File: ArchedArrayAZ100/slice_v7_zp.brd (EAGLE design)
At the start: 196.4 x 249.7 mm, 118 parts

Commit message: added slice_v7 ArchedArray with 4 layers
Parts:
- removed F1: (no value), ZacksLib2:LITTLEFUSE_111_501
- moved U$1 8.00 mm to (140.0, 249.0)
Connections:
- removed net N$284: F1.P2_1, F1.P2_2, U$1.P$2
- net VCC: now also U$1.P$2; no longer F1.P1_1, F1.P1_2
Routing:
- net VCC: track 1271.0 -> 17.6 mm, vias 24 -> 1
- net N$284: track 11.3 -> 0.00 mm
- added copper zone on layer 2, net VCC

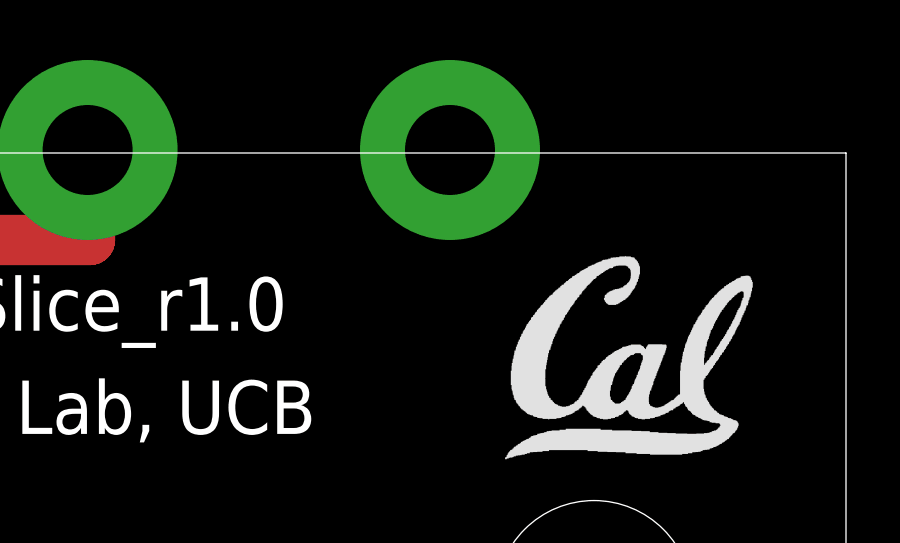
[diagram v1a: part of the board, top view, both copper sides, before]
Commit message: ArchedArray before moving board 6
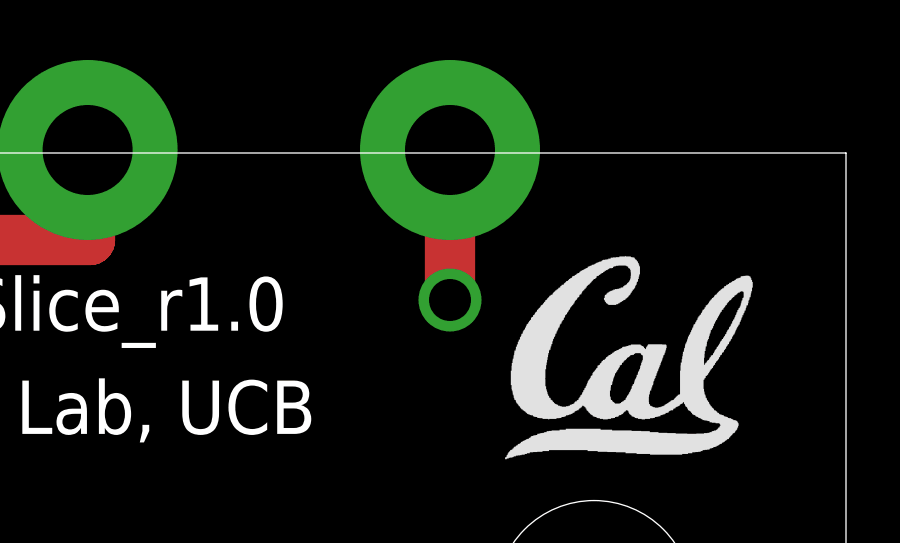
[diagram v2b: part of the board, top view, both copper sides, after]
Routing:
- net VCC: track 17.6 -> 78.7 mm
- net GND: track 617.8 -> 630.8 mm, vias 16 -> 17
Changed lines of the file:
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@@
 <wire x1="128" y1="246" x2="114.5" y2="246" width="1.6764" layer="1"/>
 <via x="114.5" y="246" extent="1-2" drill="1.4"/>
-<wire x1="114.5" y1="246" x2="114.5" y2="245" width="1.6764" layer="2"/>
+<wire x1="111" y1="226.365" x2="115.5" y2="226.365" width="1.6764" layer="2"/>
+<wire x1="115.5" y1="226.365" x2="115.5" y2="224.5" width="1.6764" layer="2"/>
+<wire x1="115.5" y1="224.5" x2="114.5" y2="224.5" width="1.6764" layer="2"/>
+<wire x1="114.5" y1="224.5" x2="114.5" y2="220" width="1.6764" layer="2"/>
+<wire x1="114.5" y1="220" x2="106" y2="220" width="1.6764" layer="2"/>
+<wire x1="106" y1="220" x2="106" y2="219.635" width="1.6764" layer="2"/>
+<wire x1="111" y1="242.365" x2="111" y2="242.5" width="1.6764" layer="2"/>
+<wire x1="111" y1="242.5" x2="114.5" y2="242.5" width="1.6764" layer="2"/>
+<wire x1="114.5" y1="242.5" x2="114.5" y2="246" width="1.6764" layer="2"/>
+<wire x1="111" y1="234.365" x2="114.5" y2="234.365" width="1.6764" layer="2"/>
+<wire x1="114.5" y1="234.365" x2="114.5" y2="242.5" width="1.6764" layer="2"/>
+<wire x1="111" y1="226.365" x2="114.5" y2="226.365" width="1.6764" layer="2"/>
+<wire x1="114.5" y1="226.365" x2="114.5" y2="234.365" width="1.6764" layer="2"/>
 <wire x1="62.635" y1="182" x2="62.635" y2="188.5" width="0" layer="19" extent="1-1"/>
 <wire x1="66.635" y1="194.5" x2="62.635" y2="188.5" width="0" layer="19" extent="1-1"/>
@@
 <wire x1="94" y1="219.635" x2="88" y2="218.365" width="0" layer="19" extent="1-1"/>
 <wire x1="100" y1="219.635" x2="94" y2="219.635" width="0" layer="19" extent="1-1"/>
-<wire x1="106" y1="219.635" x2="100" y2="219.635" width="0" layer="19" extent="1-1"/>
-<wire x1="105" y1="226.365" x2="106" y2="219.635" width="0" layer="19" extent="1-1"/>
-<wire x1="111" y1="226.365" x2="105" y2="226.365" width="0" layer="19" extent="1-1"/>
+<wire x1="106" y1="220" x2="100" y2="219.635" width="0" layer="19" extent="1-2"/>
+<wire x1="106" y1="242.365" x2="111" y2="242.365" width="0" layer="19" extent="1-1"/>
+<wire x1="105.5" y1="234.365" x2="111" y2="234.365" width="0" layer="19" extent="1-1"/>
 <wire x1="99" y1="226.365" x2="105" y2="226.365" width="0" layer="19" extent="1-1"/>
 <wire x1="93" y1="226.365" x2="99" y2="226.365" width="0" layer="19" extent="1-1"/>
@@
 <wire x1="63" y1="218.865" x2="69" y2="218.865" width="0" layer="19" extent="1-1"/>
 <wire x1="57" y1="219.865" x2="63" y2="218.865" width="0" layer="19" extent="1-1"/>
-<wire x1="111" y1="234.365" x2="111" y2="226.365" width="0" layer="19" extent="1-1"/>
-<wire x1="105.5" y1="234.365" x2="111" y2="234.365" width="0" layer="19" extent="1-1"/>
-<wire x1="111" y1="242.365" x2="111" y2="234.365" width="0" layer="19" extent="1-1"/>
-<wire x1="114.5" y1="245" x2="111" y2="242.365" width="0" layer="19" extent="1-2"/>
-<wire x1="106" y1="242.365" x2="111" y2="242.365" width="0" layer="19" extent="1-1"/>
 <wire x1="97.75" y1="243.5" x2="106" y2="242.365" width="0" layer="19" extent="1-1"/>
 <wire x1="93.48" y1="241.818" x2="97.75" y2="243.5" width="0" layer="19" extent="1-16"/>
@@
 <wire x1="13.096" y1="166.662" x2="32.5" y2="156.635" width="0" layer="19" extent="16-16"/>
 <wire x1="15.5" y1="170.75" x2="13.096" y2="166.662" width="0" layer="19" extent="1-16"/>
+<wire x1="111" y1="226.365" x2="114" y2="226.365" width="1.6764" layer="2"/>
+<wire x1="114" y1="226.365" x2="114" y2="234.5" width="1.6764" layer="2"/>
+<wire x1="114" y1="234.5" x2="105.5" y2="234.365" width="0" layer="19" extent="1-16"/>
 </signal>
 <signal name="N$29">
@@
 <wire x1="-7.342" y1="125.856" x2="-8.4" y2="127.1" width="0" layer="19" extent="16-16"/>
 <wire x1="-25.09" y1="77.248" x2="-26.79" y2="79.19" width="0" layer="19" extent="16-16"/>
-<wire x1="140" y1="249" x2="97.8" y2="246.2" width="0" layer="19" extent="1-1"/>
+<wire x1="140" y1="249" x2="140" y2="244" width="1.6764" layer="1"/>
+<via x="140" y="244" extent="1-2" drill="1.4"/>
+<wire x1="140" y1="244" x2="133.5" y2="244" width="1.6764" layer="2"/>
+<wire x1="133.5" y1="244" x2="133.5" y2="245.5" width="1.6764" layer="2"/>
+<wire x1="133.5" y1="245.5" x2="97.8" y2="246.2" width="0" layer="19" extent="1-16"/>
 </signal>
 <signal name="N$288">

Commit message: added changes to ArchedArray board according to email
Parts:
- U$1: value 2PIN_PWR3-6-12MM -> 2PIN_PWR4-8-16MM
- moved U$1 40.6 mm to (100.5, 239.4), turned to 0 degrees
- moved D2 19.8 mm to (110.5, 208.0)
- moved D12 19.3 mm to (96.5, 208.0), turned to 90 degrees
- moved D8 19.2 mm to (82.5, 221.0), turned to 270 degrees
- moved CHIP_6 19.2 mm to (96.5, 218.5)
- moved D1 19.2 mm to (108.0, 216.0)
- moved D14 19.2 mm to (113.5, 216.0)
- moved D4 19.2 mm to (101.5, 208.0)
- moved D5 19.2 mm to (113.5, 224.0)
- moved D6 19.2 mm to (108.5, 224.0)
- moved D16 17.7 mm to (87.5, 225.5), turned to 270 degrees
- moved D13 16.7 mm to (113.5, 210.5)
- moved D10 15.6 mm to (78.5, 220.0), turned to 270 degrees
- moved C1 14.9 mm to (99.3, 229.0), turned to 180 degrees
- moved D15 14.3 mm to (91.5, 207.5)
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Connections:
- net N$1: now also D10.3; no longer D10.1
- net N$100: now also D43.3; no longer D43.1
- net N$101: now also D43.1; no longer D43.3
- net N$103: now also D44.3; no longer D44.1
- net N$104: now also D44.1; no longer D44.3
- net N$106: now also D40.3; no longer D40.1
- net N$107: now also D40.1; no longer D40.3
- net N$109: now also D35.3; no longer D35.1
- net N$11: now also D12.3; no longer D12.1
- net N$110: now also D35.1; no longer D35.3
- net N$113: now also D48.1; no longer D48.3
- net N$114: now also D48.3; no longer D48.1
- net N$115: now also D47.3; no longer D47.1
- net N$116: now also D47.1; no longer D47.3
- net N$119: now also D37.3; no longer D37.1
- net N$12: now also D12.1; no longer D12.3
- net N$121: now also D38.1; no longer D38.3
- net N$122: now also D34.3; no longer D34.1
- net N$123: now also D36.1; no longer D36.3
- net N$124: now also D36.3; no longer D36.1
- net N$125: now also D37.1; no longer D37.3
- net N$126: now also D38.3; no longer D38.1
- net N$127: now also D34.1; no longer D34.3
- net N$130: now also D41.3; no longer D41.1
- net N$131: now also D41.1; no longer D41.3
- net N$133: now also D33.3; no longer D33.1
- net N$135: now also D45.3; no longer D45.1
- net N$136: now also D45.1; no longer D45.3
- net N$139: now also D46.3; no longer D46.1
- net N$14: now also D8.3; no longer D8.1
- net N$140: now also D33.1; no longer D33.3
- net N$141: now also D46.1; no longer D46.3
- net N$142: now also D58.3; no longer D58.1
- net N$144: now also D55.3; no longer D55.1
- net N$145: now also D55.1; no longer D55.3
- net N$147: now also D59.3; no longer D59.1
- net N$148: now also D59.1; no longer D59.3
- net N$15: now also D8.1; no longer D8.3
- net N$150: now also D60.3; no longer D60.1
- net N$151: now also D60.1; no longer D60.3
- net N$153: now also D56.3; no longer D56.1
- net N$154: now also D56.1; no longer D56.3
- net N$156: now also D51.3; no longer D51.1
- net N$157: now also D51.1; no longer D51.3
- net N$160: now also D64.1; no longer D64.3
- net N$161: now also D64.3; no longer D64.1
- net N$162: now also D63.3; no longer D63.1
- net N$163: now also D63.1; no longer D63.3
- net N$166: now also D53.3; no longer D53.1
- net N$168: now also D54.1; no longer D54.3
- net N$169: now also D50.3; no longer D50.1
- net N$17: now also D3.1; no longer D3.3
- net N$170: now also D52.1; no longer D52.3
- net N$171: now also D52.3; no longer D52.1
- net N$172: now also D53.1; no longer D53.3
- net N$173: now also D54.3; no longer D54.1
- net N$174: now also D50.1; no longer D50.3
- net N$177: now also D57.3; no longer D57.1
- net N$178: now also D57.1; no longer D57.3
- net N$180: now also D49.3; no longer D49.1
- net N$182: now also D61.3; no longer D61.1
- net N$183: now also D61.1; no longer D61.3
- net N$186: now also D62.3; no longer D62.1
- net N$187: now also D49.1; no longer D49.3
- net N$188: now also D62.1; no longer D62.3
- net N$189: now also D74.3; no longer D74.1
- net N$191: now also D71.3; no longer D71.1
- net N$192: now also D71.1; no longer D71.3
- net N$194: now also D75.3; no longer D75.1
- net N$195: now also D75.1; no longer D75.3
- net N$197: now also D76.3; no longer D76.1
- net N$198: now also D76.1; no longer D76.3
- net N$2: now also D3.3; no longer D3.1
- net N$20: now also D16.1; no longer D16.3
- net N$200: now also D72.3; no longer D72.1
- net N$201: now also D72.1; no longer D72.3
- net N$203: now also D67.3; no longer D67.1
- net N$204: now also D67.1; no longer D67.3
- net N$207: now also D80.1; no longer D80.3
- net N$208: now also D80.3; no longer D80.1
- net N$209: now also D79.3; no longer D79.1
- net N$21: now also D16.3; no longer D16.1
- net N$210: now also D79.1; no longer D79.3
- net N$213: now also D69.3; no longer D69.1
- net N$215: now also D70.1; no longer D70.3
- net N$216: now also D66.3; no longer D66.1
- net N$217: now also D68.1; no longer D68.3
- net N$218: now also D68.3; no longer D68.1
- net N$219: now also D69.1; no longer D69.3
- net N$22: now also D15.3; no longer D15.1
- net N$220: now also D70.3; no longer D70.1
- net N$221: now also D66.1; no longer D66.3
- net N$224: now also D73.3; no longer D73.1
- net N$225: now also D73.1; no longer D73.3
- net N$227: now also D65.3; no longer D65.1
- net N$229: now also D77.3; no longer D77.1
- net N$23: now also D15.1; no longer D15.3
- net N$230: now also D77.1; no longer D77.3
- net N$233: now also D78.3; no longer D78.1
- net N$234: now also D65.1; no longer D65.3
- net N$235: now also D78.1; no longer D78.3
- net N$236: now also D90.3; no longer D90.1
- net N$238: now also D87.3; no longer D87.1
- net N$239: now also D87.1; no longer D87.3
- net N$241: now also D91.3; no longer D91.1
- net N$242: now also D91.1; no longer D91.3
- net N$244: now also D92.3; no longer D92.1
- net N$245: now also D92.1; no longer D92.3
- net N$247: now also D88.3; no longer D88.1
- net N$248: now also D88.1; no longer D88.3
- net N$25: now also D9.1; no longer D9.3
- net N$250: now also D83.3; no longer D83.1
- net N$251: now also D83.1; no longer D83.3
- net N$254: now also D96.1; no longer D96.3
- net N$255: now also D96.3; no longer D96.1
- net N$256: now also D95.3; no longer D95.1
- net N$257: now also D95.1; no longer D95.3
- net N$26: now also D4.1; no longer D4.3
- net N$260: now also D85.3; no longer D85.1
- net N$262: now also D86.1; no longer D86.3
- net N$263: now also D82.3; no longer D82.1
- net N$264: now also D84.1; no longer D84.3
- net N$265: now also D84.3; no longer D84.1
- net N$266: now also D85.1; no longer D85.3
- net N$267: now also D86.3; no longer D86.1
- net N$268: now also D82.1; no longer D82.3
- net N$27: now also D4.3; no longer D4.1
- net N$271: now also D89.3; no longer D89.1
- net N$272: now also D89.1; no longer D89.3
- net N$274: now also D81.3; no longer D81.1
- net N$276: now also D93.3; no longer D93.1
- net N$277: now also D93.1; no longer D93.3
- net N$28: now also D5.1; no longer D5.3
- net N$280: now also D94.3; no longer D94.1
- net N$281: now also D81.1; no longer D81.3
- net N$282: now also D94.1; no longer D94.3
- net N$288: now also D90.1; no longer D90.3
- net N$289: now also D42.1; no longer D42.3
- net N$290: now also D26.1; no longer D26.3
- net N$293: now also D10.1; no longer D10.3
- net N$298: now also D74.1; no longer D74.3
- net N$300: now also D58.1; no longer D58.3
- net N$31: now also D5.3; no longer D5.1
- net N$33: now also D6.1; no longer D6.3
- net N$34: now also D1.3; no longer D1.1
- net N$35: now also D2.3; no longer D2.1
- net N$36: now also D14.1; no longer D14.3
- net N$38: now also D6.3; no longer D6.1
- net N$39: now also D13.3; no longer D13.1
- net N$4: now also D7.3; no longer D7.1
- net N$40: now also D13.1; no longer D13.3
- net N$42: now also D2.1; no longer D2.3
- net N$45: now also D26.3; no longer D26.1
- net N$47: now also D14.3; no longer D14.1
- net N$49: now also D1.1; no longer D1.3
- net N$5: now also D7.1; no longer D7.3
- net N$50: now also D23.3; no longer D23.1
- net N$51: now also D23.1; no longer D23.3
- net N$53: now also D27.3; no longer D27.1
- net N$54: now also D27.1; no longer D27.3
- net N$56: now also D28.3; no longer D28.1
- net N$57: now also D28.1; no longer D28.3
- net N$59: now also D24.3; no longer D24.1
- net N$60: now also D24.1; no longer D24.3
- net N$62: now also D19.3; no longer D19.1
- net N$63: now also D19.1; no longer D19.3
- net N$66: now also D32.1; no longer D32.3
- net N$67: now also D32.3; no longer D32.1
- net N$68: now also D31.3; no longer D31.1
- net N$69: now also D31.1; no longer D31.3
- net N$7: now also D11.3; no longer D11.1
- net N$72: now also D21.3; no longer D21.1
- net N$74: now also D22.1; no longer D22.3
- net N$75: now also D18.3; no longer D18.1
- net N$76: now also D20.1; no longer D20.3
- net N$77: now also D20.3; no longer D20.1
- net N$78: now also D21.1; no longer D21.3
- net N$79: now also D22.3; no longer D22.1
- net N$8: now also D9.3; no longer D9.1
- net N$80: now also D18.1; no longer D18.3
- net N$83: now also D25.3; no longer D25.1
- net N$84: now also D25.1; no longer D25.3
- net N$86: now also D17.3; no longer D17.1
- net N$88: now also D29.3; no longer D29.1
- net N$89: now also D29.1; no longer D29.3
- net N$9: now also D11.1; no longer D11.3
- net N$92: now also D30.3; no longer D30.1
- net N$93: now also D17.1; no longer D17.3
- net N$94: now also D30.1; no longer D30.3
- net N$95: now also D42.3; no longer D42.1
- net N$97: now also D39.3; no longer D39.1
- net N$98: now also D39.1; no longer D39.3
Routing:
- net VCC: track 78.7 -> 1176.0 mm, vias 1 -> 18
- net GSCLK: track 81.2 -> 347.2 mm, vias 2 -> 11
- net GND: track 630.8 -> 554.4 mm, vias 17 -> 14
- net N$15: track 58.6 -> 11.1 mm
- net N$14: track 58.7 -> 11.3 mm
- net N$20: track 52.2 -> 5.80 mm
- net N$16: track 56.4 -> 12.1 mm
- net N$21: track 50.7 -> 7.83 mm
- net N$285: track 182.7 -> 140.1 mm, vias 3 -> 2
- net N$19: track 48.4 -> 8.61 mm
- net N$1: track 55.0 -> 20.6 mm
- net N$293: track 56.3 -> 22.6 mm
- net N$3: track 52.7 -> 19.8 mm
- net N$5: track 34.6 -> 13.6 mm
- net N$30: track 30.2 -> 9.67 mm
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- removed copper zone on layer 2, net VCC
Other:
- board size 196.4 x 249.7 mm -> 196.8 x 247.8 mm
- board text removed: "7A Fuse"
